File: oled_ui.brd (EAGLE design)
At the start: 81.4 x 19.2 mm, 42 parts, among them IC1 74HC14D

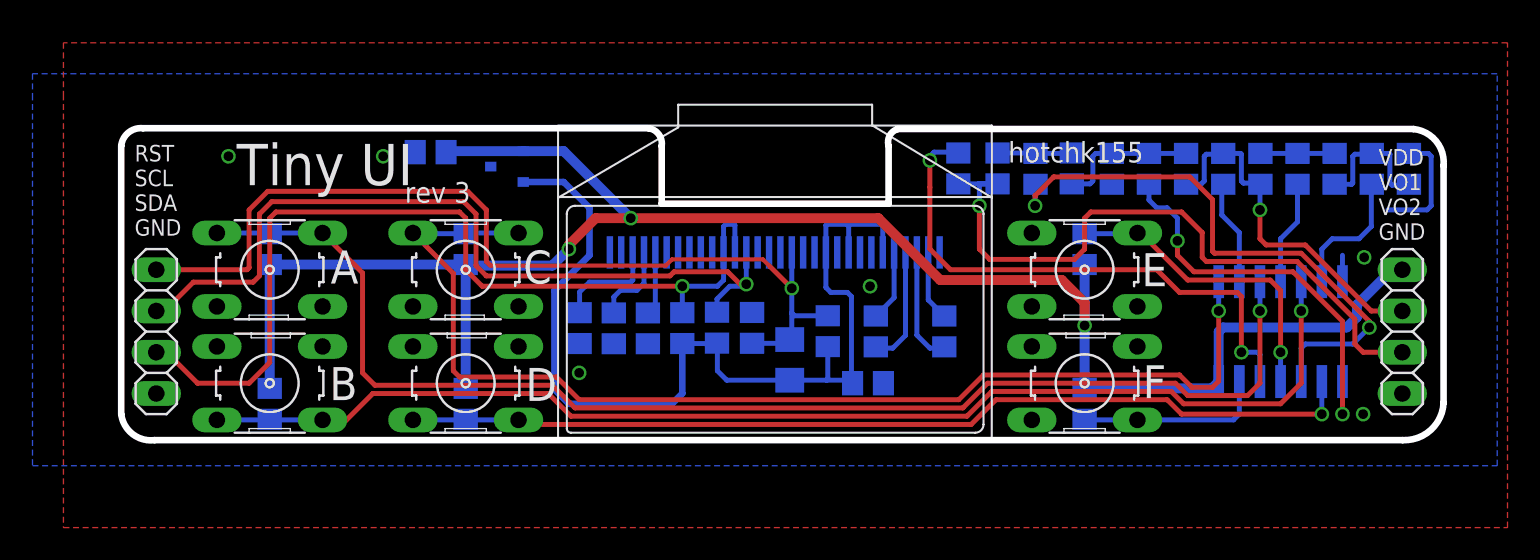
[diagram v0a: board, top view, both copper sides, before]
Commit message: pcb rev 4
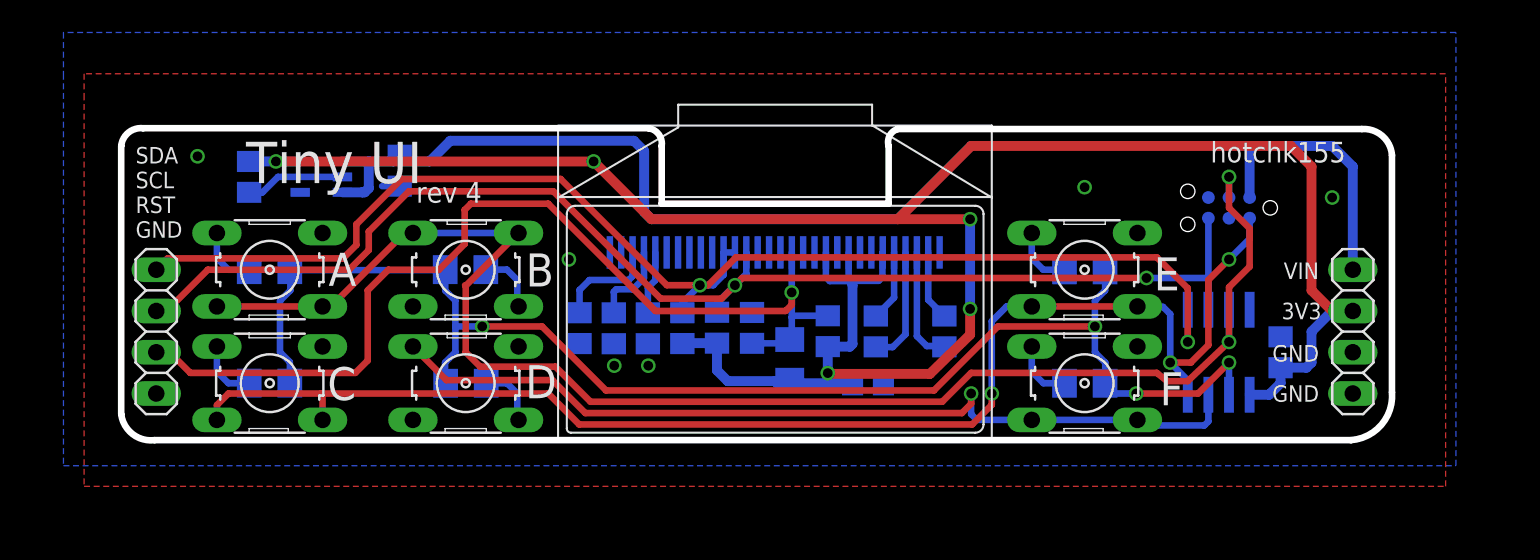
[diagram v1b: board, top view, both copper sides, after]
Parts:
- removed 1A, 1B, 2A, 2B, 3A, 3B, 4A, 4B, 5B, 6B, 7B, 8B, J1, R3, R4, R5, R6, R7, R8: (no value), rcl:R0805
- removed C2: (no value), rcl:C0805
- added C10, C9: (no value), rcl:C0805
- added C8: 100n, rcl:C0805
- added ICSP: (no value), tag-connect:TC2030-MCP-NL
- added U$3, U$4, U$5, U$6, U$7, U$8: 0805DIODE, jasons_stuff:0805DIODE
- C1, C5, C6: value (none) -> 1u
- C3: value (none) -> 2u2
- C4: value (none) -> 4u7
- C7: value (none) -> 100n?
- IC1: value 74HC14D -> PIC12F1822SO08; device 74xx-eu:SO14 -> jasons_stuff:SO08
- IC2: value (none) -> MIC5504-2.8YM5-TR; device microbuilder:SOT23-R -> jason_eagle6:SOT23-5
- R1: value (none) -> 390k
- R10, R9: value (none) -> 4k7
- R2: value (none) -> 10k?
- moved B 13.9 mm to (24.1, 12.7)
- moved C 13.9 mm to (12.1, 5.71)
- moved IC2 11.4 mm to (15.2, 18.4)
- moved IC1 4.02 mm to (70.5, 7.62), turned to 0 degrees
- moved JP2 3.05 mm to (78.7, 8.89)
- turned F to 0 degrees
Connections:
- removed net BUTTONS_OUT1: 4A.1, 8B.1, JP2.3
- removed net BUTTONS_OUT2: 2A.1, 4B.1, J1.2, JP2.2
- removed net N$13: E.1, E.2, IC1.11, R4.1
- removed net N$15: 3B.2, IC1.4
- removed net N$16: 2B.2, IC1.6
- removed net N$17: 1A.2, 1B.1, 2B.1
- removed net N$18: 1A.1, 2A.2, 3B.1
- removed net N$20: 6B.2, IC1.8
- removed net N$21: 3A.2, 5B.1, 6B.1, J1.1
- removed net N$22: 7B.2, IC1.10
- removed net N$23: 3A.1, 4A.2, 7B.1
- removed net N$24: 8B.2, IC1.12
- new net KEYA: IC1.2, U$3.A, U$4.A, U$5.A, U$6.C, U$7.C, U$8.C
- new net KEYB: D.3, D.4, F.3, F.4, IC1.3
- new net KEYC: C.3, C.4, E.3, E.4, IC1.4, ICSP.1
- new net KEYD: A.3, A.4, B.3, B.4, IC1.7, ICSP.4
- net 3V3: now also C10.1, C8.1, IC1.1, IC2.5, JP2.2; no longer IC2.2
- net 5V: now also C9.1, IC2.3, ICSP.2; no longer C2.1, IC1.14, R3.2, R4.2, R5.2, R6.2, R7.2, R8.2
- net GND: now also C10.2, C8.2, C9.2, IC1.8, IC2.2, ICSP.3, JP2.3; no longer 1B.2, 5B.2, A.3, A.4, B.3, B.4, C.3, C.4, C2.2, D.3, D.4, E.3, E.4, F.3, F.4, IC1.7, IC2.3
- net N$11: now also E.1, U$4.C; no longer C.1, C.2, IC1.1, R6.1
- net N$12: now also B.1, U$5.C; no longer D.1, D.2, IC1.9, R5.1
- net N$14: now also A.1, U$8.A; no longer F.1, F.2, IC1.13, R3.1
- net N$5: now also F.1, U$3.C; no longer B.1, B.2, IC1.5, R8.1
- net N$7: now also D.1, U$6.A; no longer 4B.2, IC1.2
- net N$9: now also C.1, U$7.A; no longer A.1, A.2, IC1.3, R7.1
- net RST: now also JP1.3; no longer JP1.1
- net SCL: now also IC1.6, ICSP.5
- net SDA: now also IC1.5, JP1.1; no longer JP1.3
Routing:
- net KEYD: track 0.00 -> 93.8 mm, vias 0 -> 2
- net KEYC: track 0.00 -> 85.6 mm, vias 0 -> 3
- net KEYA: track 0.00 -> 85.4 mm, vias 0 -> 4
- net 3V3: track 61.0 -> 143.3 mm, vias 0 -> 5
- net N$9: track 79.8 -> 3.84 mm, vias 1 -> 0
- net N$5: track 75.8 -> 3.86 mm, vias 1 -> 0
- net N$11: track 71.1 -> 3.86 mm, vias 1 -> 0
- net N$12: track 59.1 -> 3.86 mm, vias 1 -> 0
- net KEYB: track 0.00 -> 54.8 mm, vias 0 -> 1
- net BUTTONS_OUT1: track 41.6 -> 0.00 mm, vias 1 -> 0
- net N$22: track 35.7 -> 0.00 mm, vias 2 -> 0
- net N$24: track 34.3 -> 0.00 mm, vias 2 -> 0
- net 5V: track 115.9 -> 82.8 mm, vias 3 -> 0
- net SCL: track 50.5 -> 81.8 mm, vias 1 -> 2
- net SDA: track 56.6 -> 82.0 mm, vias 1 -> 2
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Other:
- board size 81.4 x 19.2 mm -> 78.2 x 19.2 mm
- board text added: "3V3"
- board text added: "GND"
- board text added: "SDA SCL RST GND"
- board text added: "VIN"
- board text added: "rev 4"
- board text removed: "RST SCL SDA GND"
- board text removed: "VDD VO1 VO2 GND"
- board text removed: "rev 3"
